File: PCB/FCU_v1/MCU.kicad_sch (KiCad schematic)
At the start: 49 parts, among them J3 Conn_01x05_Pin, SW1 SW_SPDT, U10 SN65HVD232, U2 STM32F412RETx, U3 W25Q128JVSIM, Y2 16MHz

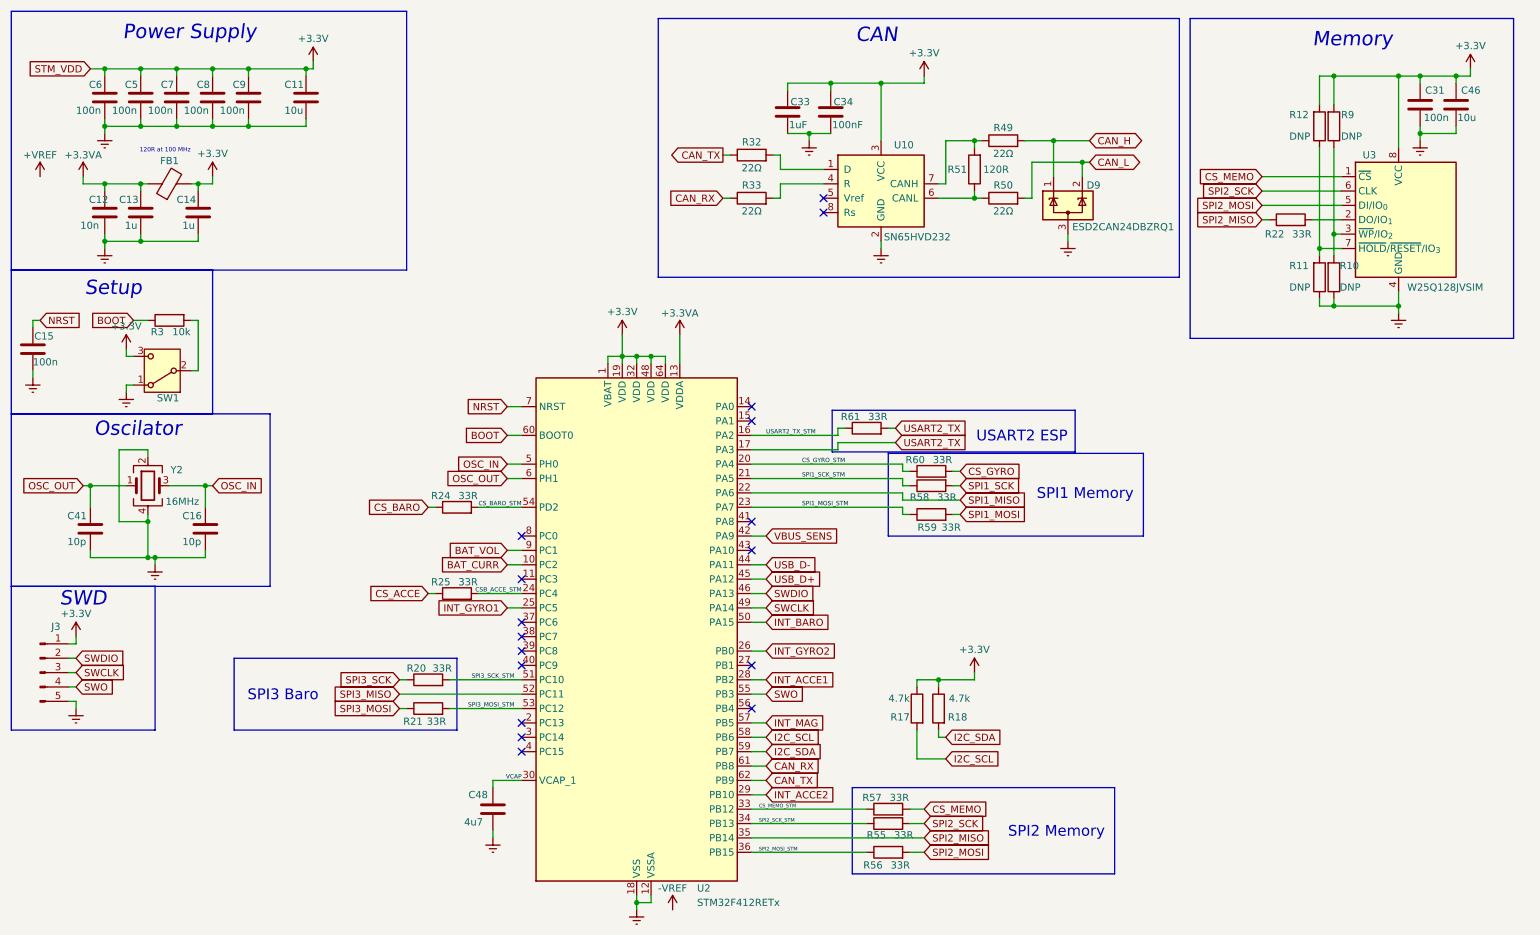
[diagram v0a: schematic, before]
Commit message: Layout update
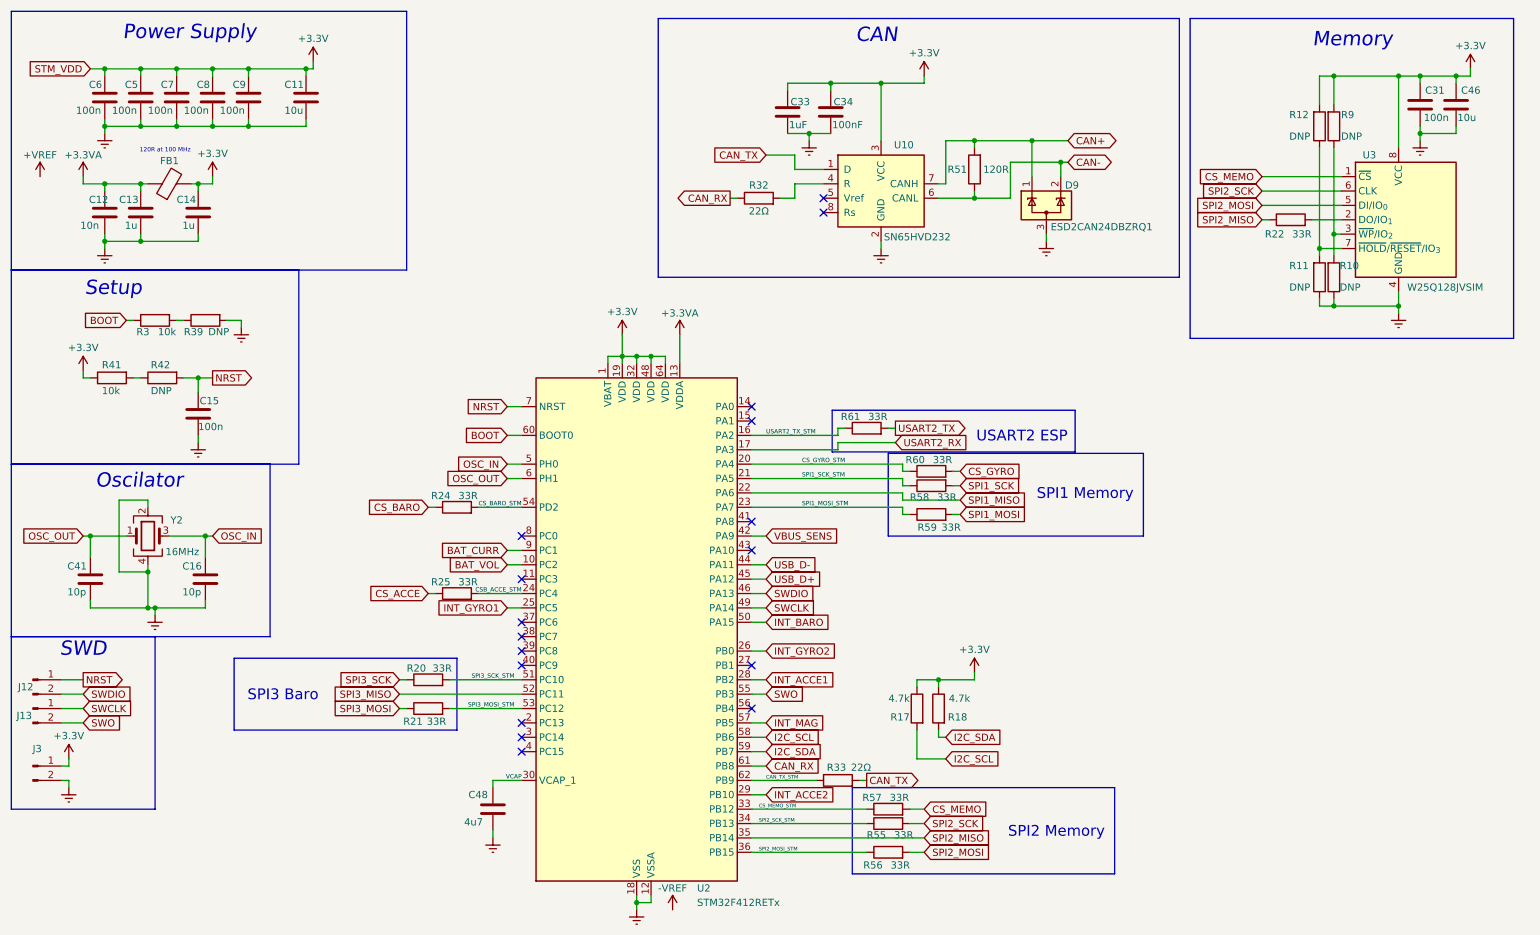
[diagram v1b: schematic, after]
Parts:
- removed J3: Conn_01x05_Pin, Connector_PinHeader_2.54mm:PinHeader_1x05_P2.54mm_Vertical, symbol Connector:Conn_01x05_Pin
- removed R49, R50: 22Ω, Resistor_SMD:R_0603_1608Metric, symbol Device:R
- removed SW1: SW_SPDT, symbol Switch:SW_SPDT
- added J12, J13, J3: Conn_01x02_Pin, Connector_PinHeader_2.54mm:PinHeader_1x02_P2.54mm_Vertical, symbol Connector:Conn_01x02_Pin
- added R39, R42: DNP, Resistor_SMD:R_0201_0603Metric, symbol Device:R
- added R41: 10k, Resistor_SMD:R_0603_1608Metric, symbol Device:R
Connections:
- net CAN_H is gone; now on net CAN+: D9.1 (K)
- net CAN_L is gone; now on net CAN-: D9.2 (K)
- net +3.3V: now also J3.1 (Pin_1), R41.1
- net BAT_CURR: now also U2.9 (PC1); no longer U2.10 (PC2)
- net BAT_VOL: now also U2.10 (PC2); no longer U2.9 (PC1)
- net CAN_RX: now also R32.1; no longer R33.1
- net CAN_TX: now also R33.2, U10.1 (D); no longer R32.1, U2.62 (PB9)
- net GND: now also J3.2 (Pin_2), R39.2
- net NRST: now also J12.1 (Pin_1), R42.2
- net SWCLK: now also J13.1 (Pin_1)
- net SWDIO: now also J12.2 (Pin_2)
- net SWO: now also J13.2 (Pin_2)
- net USART2_TX: no longer U2.17 (PA3)
- net at R3.2: now also R39.1
- net CAN-: now reaches R51.1, U10.6 (CANL)
- net CAN+: now reaches R51.2, U10.7 (CANH)
- net at U10.4 (R): now also R32.2; no longer R33.2
- new net: R41.2, R42.1
- new net CAN_TX_STM: R33.1, U2.62 (PB9)
- new net USART2_RX: U2.17 (PA3)
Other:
- moved on the sheet: C15, C16, C41, D9, R3, R32, Y2

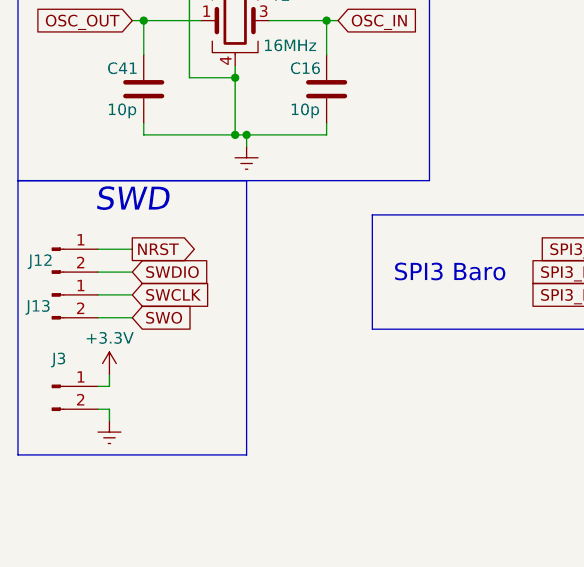
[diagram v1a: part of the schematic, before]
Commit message: Layout update
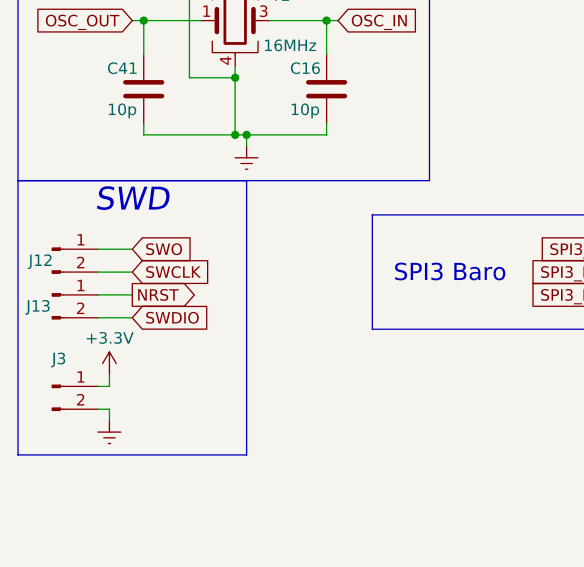
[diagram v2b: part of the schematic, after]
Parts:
- R42: footprint Resistor_SMD:R_0201_0603Metric -> Resistor_SMD:R_0402_1005Metric
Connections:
- net NRST: now also J13.1 (Pin_1); no longer J12.1 (Pin_1)
- net SWCLK: now also J12.2 (Pin_2); no longer J13.1 (Pin_1)
- net SWDIO: now also J13.2 (Pin_2); no longer J12.2 (Pin_2)
- net SWO: now also J12.1 (Pin_1); no longer J13.2 (Pin_2)
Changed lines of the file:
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@@
 	(global_label "SWCLK"
 		(shape input)
-		(at 29.21 137.16 0)
+		(at 29.21 134.62 0)
 		(fields_autoplaced yes)
 		(effects
@@
 		)
 		(property "Intersheetrefs" "${INTERSHEET_REFS}"
-			(at 38.4242 137.16 0)
+			(at 38.4242 134.62 0)
 			(effects
 				(font
@@
 	(global_label "SWDIO"
 		(shape input)
-		(at 29.21 134.62 0)
+		(at 29.21 139.7 0)
 		(fields_autoplaced yes)
 		(effects
@@
 		)
 		(property "Intersheetrefs" "${INTERSHEET_REFS}"
-			(at 38.0614 134.62 0)
+			(at 38.0614 139.7 0)
 			(effects
 				(font
@@
 	(global_label "NRST"
 		(shape output)
-		(at 29.21 132.08 0)
+		(at 29.21 137.16 0)
 		(fields_autoplaced yes)
 		(effects
@@
 		)
 		(property "Intersheetrefs" "${INTERSHEET_REFS}"
-			(at 36.9728 132.08 0)
+			(at 36.9728 137.16 0)
 			(effects
 				(font
@@
 	(global_label "SWO"
 		(shape input)
-		(at 29.21 139.7 0)
+		(at 29.21 132.08 0)
 		(fields_autoplaced yes)
 		(effects
@@
 		)
 		(property "Intersheetrefs" "${INTERSHEET_REFS}"
-			(at 36.1866 139.7 0)
+			(at 36.1866 132.08 0)
 			(effects
 				(font
@@
 			)
 		)
-		(property "Footprint" "Resistor_SMD:R_0201_0603Metric"
+		(property "Footprint" "Resistor_SMD:R_0402_1005Metric"
 			(at 43.18 76.962 90)
 			(effects
